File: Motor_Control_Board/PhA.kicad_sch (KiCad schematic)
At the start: 39 parts, among them J10 C, J2 A, J9 B, Q1 CSD18540Q5B, Q2 CSD18540Q5B, Q3 CSD18540Q5B, Q4 CSD18540Q5B, Q5 CSD18540Q5B, Q6 CSD18540Q5B, U6 INA180B3, U7 INA180B3, U8 INA180B3

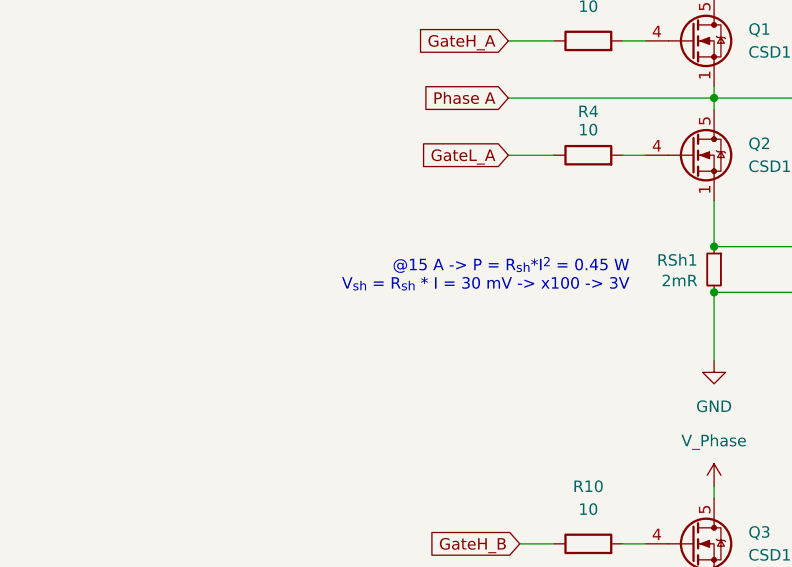
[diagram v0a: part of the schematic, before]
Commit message: Minor updates: V0.9
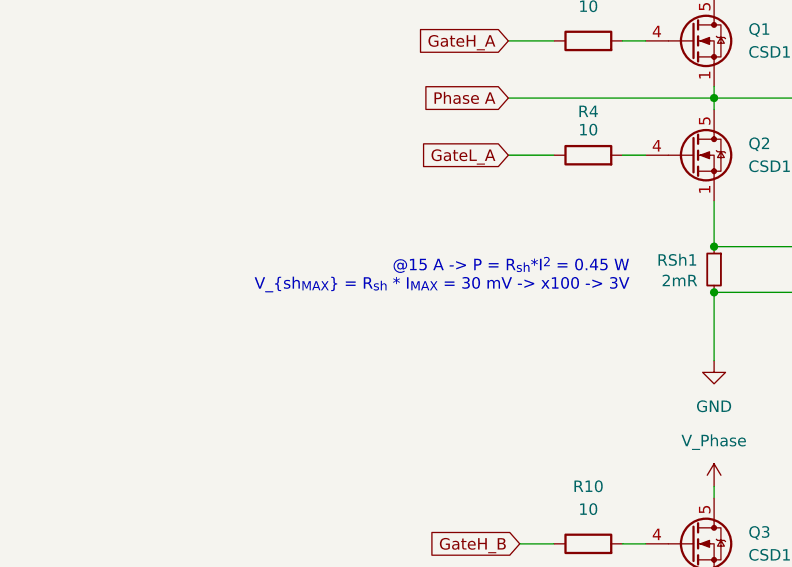
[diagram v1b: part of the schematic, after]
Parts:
- C46, C47, C49, C50, C52, C53: PartNum (none) -> 885012005018
- Q1, Q2, Q3, Q4, Q5, Q6: PartNum (none) -> CSD18540Q5B
- U6, U7, U8: PartNum (none) -> INA180B3QDBVRQ1
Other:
- note added: "@15 A -> P = R_{sh}*I^{2} = 0.45 W V_{sh_{MAX}} = R_{sh} * I_{MAX} = 30 mV -> x100 -> 3V"
- note removed: "@15 A -> P = R_{sh}*I^{2} = 0.45 W V_{sh} = R_{sh} * I = 30 mV -> x100 -> 3V"
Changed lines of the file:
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@@
 		)
 	)
-	(text "@15 A -> P = R_{sh}*I^{2} = 0.45 W\nV_{sh} = R_{sh} * I = 30 mV -> x100 -> 3V\n"
+	(text "@15 A -> P = R_{sh}*I^{2} = 0.45 W\nV_{sh_{MAX}} = R_{sh} * I_{MAX} = 30 mV -> x100 -> 3V\n"
 		(exclude_from_sim no)
 		(at 66.802 51.562 0)
@@
 			)
 		)
+		(property "PartNum" "CSD18540Q5B"
+			(at 73.66 93.98 0)
+			(effects
+				(font
+					(size 1.27 1.27)
+				)
+				(hide yes)
+			)
+		)
 		(pin "5"
 		)
@@
 			)
 		)
+		(property "PartNum" "INA180B3QDBVRQ1"
+			(at 101.6 50.8 0)
+			(effects
+				(font
+					(size 1.27 1.27)
+				)
+				(hide yes)
+			)
+		)
 		(pin "1"
 		)
@@
 			)
 		)
+		(property "PartNum" "INA180B3QDBVRQ1"
+			(at 101.6 162.56 0)
+			(effects
+				(font
+					(size 1.27 1.27)
+				)
+				(hide yes)
+			)
+		)
 		(pin "1"
 		)
@@
 			)
 		)
+		(property "PartNum" "CSD18540Q5B"
+			(at 73.66 25.4 0)
+			(effects
+				(font
+					(size 1.27 1.27)
+				)
+				(hide yes)
+			)
+		)
 		(pin "5"
 		)
@@
 			)
 		)
+		(property "PartNum" "885012005018"
+			(at 120.65 109.22 0)
+			(effects
+				(font
+					(size 1.27 1.27)
+				)
+				(hide yes)
+			)
+		)
 		(pin "1"
 		)
@@
 			)
 		)
+		(property "PartNum" "CSD18540Q5B"
+			(at 73.66 137.16 0)
+			(effects
+				(font
+					(size 1.27 1.27)
+				)
+				(hide yes)
+			)
+		)
 		(pin "5"
 		)
@@
 			)
 		)
+		(property "PartNum" "885012005018"
+			(at 146.05 54.61 0)
+			(effects
+				(font
+					(size 1.27 1.27)
+				)
+				(hide yes)
+			)
+		)
 		(pin "1"
 		)
@@
 			)
 		)
+		(property "PartNum" "CSD18540Q5B"
+			(at 73.66 81.28 0)
+			(effects
+				(font
+					(size 1.27 1.27)
+				)
+				(hide yes)
+			)
+		)
 		(pin "5"
 		)
@@
 			)
 		)
+		(property "PartNum" "885012005018"
+			(at 120.65 166.37 0)
+			(effects
+				(font
+					(size 1.27 1.27)
+				)
+				(hide yes)
+			)
+		)
 		(pin "1"
 		)
@@
 			)
 		)
+		(property "PartNum" "885012005018"
+			(at 120.65 54.61 0)
+			(effects
+				(font
+					(size 1.27 1.27)
+				)
+				(hide yes)
+			)
+		)
 		(pin "1"
 		)
@@
 			)
 		)
+		(property "PartNum" "CSD18540Q5B"
+			(at 73.66 38.1 0)
+			(effects
+				(font
+					(size 1.27 1.27)
+				)
+				(hide yes)
+			)
+		)
 		(pin "5"
 		)
@@
 			)
 		)
+		(property "PartNum" "885012005018"
+			(at 148.59 110.49 0)
+			(effects
+				(font
+					(size 1.27 1.27)
+				)
+				(hide yes)
+			)
+		)
 		(pin "1"
 		)
@@
 			)
 		)
+		(property "PartNum" "885012005018"
+			(at 147.32 166.37 0)
+			(effects
+				(font
+					(size 1.27 1.27)
+				)
+				(hide yes)
+			)
+		)
 		(pin "1"
 		)
@@
 			)
 		)
+		(property "PartNum" "CSD18540Q5B"
+			(at 73.66 149.86 0)
+			(effects
+				(font
+					(size 1.27 1.27)
+				)
+				(hide yes)
+			)
+		)
 		(pin "5"
 		)
@@
 			(at 101.6 105.41 0)
 			(effects
+				(font
+					(size 1.27 1.27)
+				)
+				(hide yes)
+			)
+		)
+		(property "PartNum" "INA180B3QDBVRQ1"
+			(at 101.6 105.41 0)
+			(effects
